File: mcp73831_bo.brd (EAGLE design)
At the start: 160 x 100 mm, 9 parts, among them U1 MCP73831, X1 USBSMD

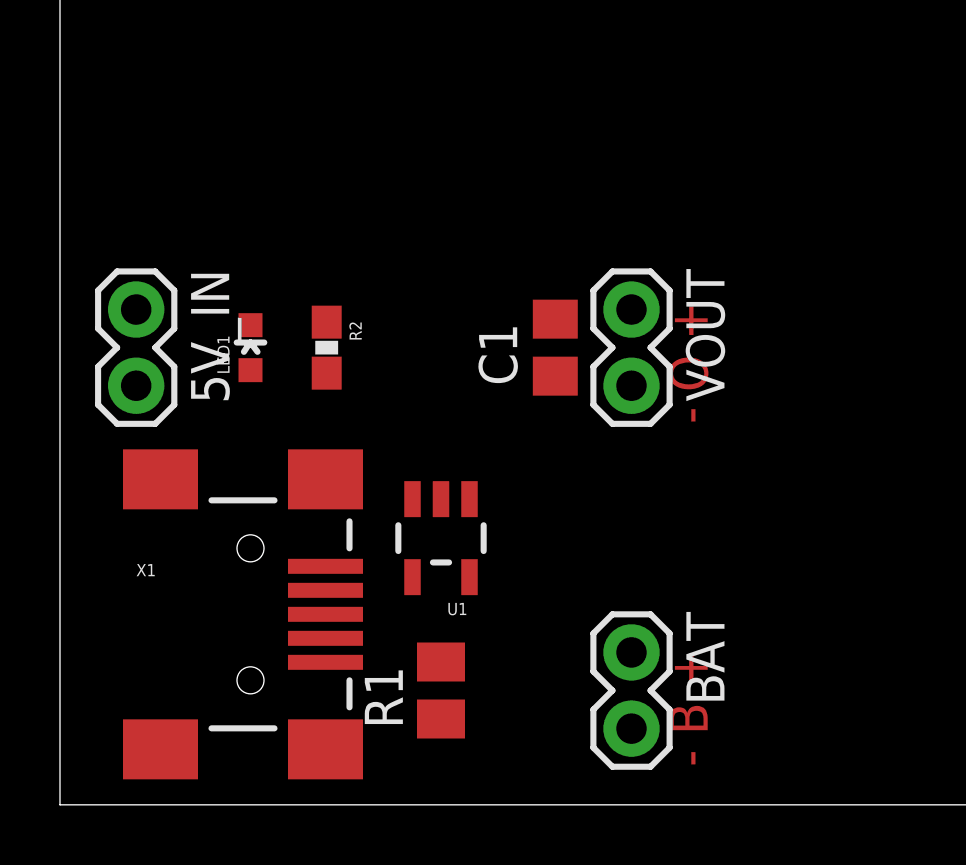
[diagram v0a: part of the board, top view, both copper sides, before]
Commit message: gndplane
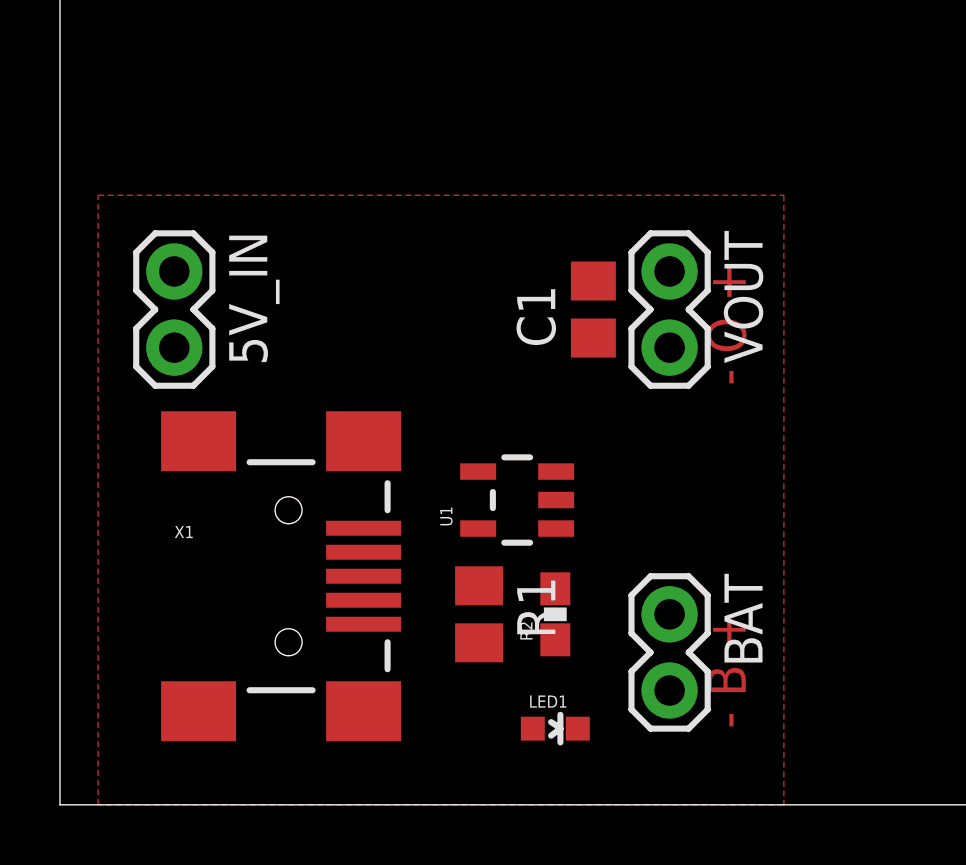
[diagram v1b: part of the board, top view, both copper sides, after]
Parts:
- moved LED1 16.3 mm to (16.5, 2.54), turned to 270 degrees
- moved R2 11.7 mm to (16.5, 6.35), turned to 90 degrees
- moved U1 2.84 mm to (15.2, 10.2), turned to 90 degrees
- moved R1 2.84 mm to (14.0, 6.35), turned to 270 degrees
- moved X1 1.80 mm to (7.62, 7.62)
- moved C1 1.80 mm to (17.8, 16.5)
- moved 5V_IN 1.80 mm to (3.81, 17.8)
- moved BAT 1.80 mm to (20.3, 6.35)
- moved VOUT 1.80 mm to (20.3, 17.8)
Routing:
- added copper zone on layer 1, net GND
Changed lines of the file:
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@@
 <wire x1="160" y1="100" x2="0" y2="100" width="0" layer="20"/>
 <wire x1="0" y1="100" x2="0" y2="0" width="0" layer="20"/>
-<text x="21.59" y="12.7" size="1.27" layer="1" rot="R90">- O +</text>
-<text x="21.59" y="1.27" size="1.27" layer="1" rot="R90">- B +</text>
+<text x="22.86" y="13.97" size="1.27" layer="1" rot="R90">- O +</text>
+<text x="22.86" y="2.54" size="1.27" layer="1" rot="R90">- B +</text>
 </plain>
 <attributes>
@@
 </autorouter>
 <elements>
-<element name="U1" library="SparkFun-PowerIC" package="SOT23-5" value="MCP73831" x="12.7" y="8.89" rot="R180"/>
-<element name="5V_IN" library="SparkFun-Connectors" package="1X02" value="" x="2.54" y="16.51" rot="R270"/>
-<element name="BAT" library="SparkFun-Connectors" package="1X02" value="" x="19.05" y="5.08" rot="R270"/>
-<element name="VOUT" library="SparkFun-Connectors" package="1X02" value="" x="19.05" y="16.51" rot="R270"/>
-<element name="X1" library="SparkFun-Connectors" package="USB-MINIB" value="USBSMD" x="6.35" y="6.35"/>
-<element name="R2" library="SparkFun-Passives" package="0603-RES" value="470" x="8.89" y="15.24" rot="R270"/>
-<element name="LED1" library="SparkFun-LED" package="LED-0603" value="" x="6.35" y="15.24"/>
-<element name="C1" library="rcl" package="C0805" value="4.7uF+" x="16.51" y="15.24" rot="R90"/>
-<element name="R1" library="rcl" package="M0805" value="2-7k" x="12.7" y="3.81" rot="R90"/>
+<element name="U1" library="SparkFun-PowerIC" package="SOT23-5" value="MCP73831" x="15.24" y="10.16" rot="R90"/>
+<element name="5V_IN" library="SparkFun-Connectors" package="1X02" value="" x="3.81" y="17.78" rot="R270"/>
+<element name="BAT" library="SparkFun-Connectors" package="1X02" value="" x="20.32" y="6.35" rot="R270"/>
+<element name="VOUT" library="SparkFun-Connectors" package="1X02" value="" x="20.32" y="17.78" rot="R270"/>
+<element name="X1" library="SparkFun-Connectors" package="USB-MINIB" value="USBSMD" x="7.62" y="7.62"/>
+<element name="R2" library="SparkFun-Passives" package="0603-RES" value="470" x="16.51" y="6.35" rot="R90"/>
+<element name="LED1" library="SparkFun-LED" package="LED-0603" value="" x="16.51" y="2.54" rot="R270"/>
+<element name="C1" library="rcl" package="C0805" value="4.7uF+" x="17.78" y="16.51" rot="R90"/>
+<element name="R1" library="rcl" package="M0805" value="2-7k" x="13.97" y="6.35" rot="R270"/>
 </elements>
 <signals>
@@
 <contactref element="C1" pad="1"/>
 <contactref element="R1" pad="2"/>
-<wire x1="16.51" y1="14.29" x2="19.05" y2="13.97" width="0" layer="19" extent="1-1"/>
-<wire x1="12.7" y1="10.1901" x2="16.51" y2="14.29" width="0" layer="19" extent="1-1"/>
-<wire x1="12.7" y1="4.76" x2="12.7" y2="10.1901" width="0" layer="19" extent="1-1"/>
-<wire x1="8.85" y1="4.75" x2="12.7" y2="4.76" width="0" layer="19" extent="1-1"/>
-<wire x1="19.05" y1="2.54" x2="12.7" y2="4.76" width="0" layer="19" extent="1-1"/>
-<wire x1="2.54" y1="13.97" x2="12.7" y2="10.1901" width="0" layer="19" extent="1-1"/>
+<polygon width="0.4064" layer="1" isolate="0.4064">
+<vertex x="1.27" y="20.32"/>
+<vertex x="24.13" y="20.32"/>
+<vertex x="24.13" y="0"/>
+<vertex x="1.27" y="0"/>
+</polygon>
 </signal>
 <signal name="5V">
@@
 <contactref element="5V_IN" pad="1"/>
 <contactref element="LED1" pad="A"/>
-<wire x1="6.35" y1="14.49" x2="2.54" y2="16.51" width="0" layer="19" extent="1-1"/>
-<wire x1="8.85" y1="7.95" x2="6.35" y2="14.49" width="0" layer="19" extent="1-1"/>
-<wire x1="11.75" y1="7.5899" x2="8.85" y2="7.95" width="0" layer="19" extent="1-1"/>
+<wire x1="10.12" y1="9.22" x2="13.9399" y2="11.11" width="0" layer="19" extent="1-1"/>
+<wire x1="15.76" y1="2.54" x2="10.12" y2="9.22" width="0" layer="19" extent="1-1"/>
+<wire x1="3.81" y1="17.78" x2="10.12" y2="9.22" width="0" layer="19" extent="1-1"/>
 </signal>
 <signal name="VBAT">
@@
 <contactref element="VOUT" pad="1"/>
 <contactref element="C1" pad="2"/>
-<wire x1="16.51" y1="16.19" x2="19.05" y2="16.51" width="0" layer="19" extent="1-1"/>
-<wire x1="11.75" y1="10.1901" x2="16.51" y2="16.19" width="0" layer="19" extent="1-1"/>
-<wire x1="19.05" y1="5.08" x2="11.75" y2="10.1901" width="0" layer="19" extent="1-1"/>
+<wire x1="17.78" y1="17.46" x2="20.32" y2="17.78" width="0" layer="19" extent="1-1"/>
+<wire x1="16.5401" y1="11.11" x2="17.78" y2="17.46" width="0" layer="19" extent="1-1"/>
+<wire x1="20.32" y1="6.35" x2="16.5401" y2="11.11" width="0" layer="19" extent="1-1"/>
 </signal>
 <signal name="N$4">
 <contactref element="U1" pad="1"/>
 <contactref element="R2" pad="2"/>
-<wire x1="8.89" y1="14.39" x2="13.65" y2="10.1901" width="0" layer="19" extent="1-1"/>
+<wire x1="16.51" y1="7.2" x2="16.5401" y2="9.21" width="0" layer="19" extent="1-1"/>
 </signal>
 <signal name="N$5">
 <contactref element="R2" pad="1"/>
 <contactref element="LED1" pad="C"/>
-<wire x1="6.35" y1="15.99" x2="8.89" y2="16.09" width="0" layer="19" extent="1-1"/>
+<wire x1="17.26" y1="2.54" x2="16.51" y2="5.5" width="0" layer="19" extent="1-1"/>
 </signal>
 <signal name="PROG">
 <contactref element="U1" pad="5"/>
 <contactref element="R1" pad="1"/>
-<wire x1="12.7" y1="2.86" x2="13.65" y2="7.5899" width="0" layer="19" extent="1-1"/>
+<wire x1="13.97" y1="7.3" x2="13.9399" y2="9.21" width="0" layer="19" extent="1-1"/>
 </signal>
 </signals>
